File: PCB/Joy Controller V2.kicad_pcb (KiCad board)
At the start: 2 copper layers, 182.7 x 66.7 mm, 24 parts, among them J1 Conn_02x16_Odd_Even, J2 JOY1, J3 JOY2, J4 USB_C_Receptacle_USB2.0_16P, SW1 SW_Push, SW10 SW_Push, SW12 RotaryEncoder_Switch_MP, SW2 SW_Push, SW3 SW_Push, SW4 SW_Push, SW5 SW_Push, SW6 SW_Push, SW7 SW_Push, SW8 SW_Push

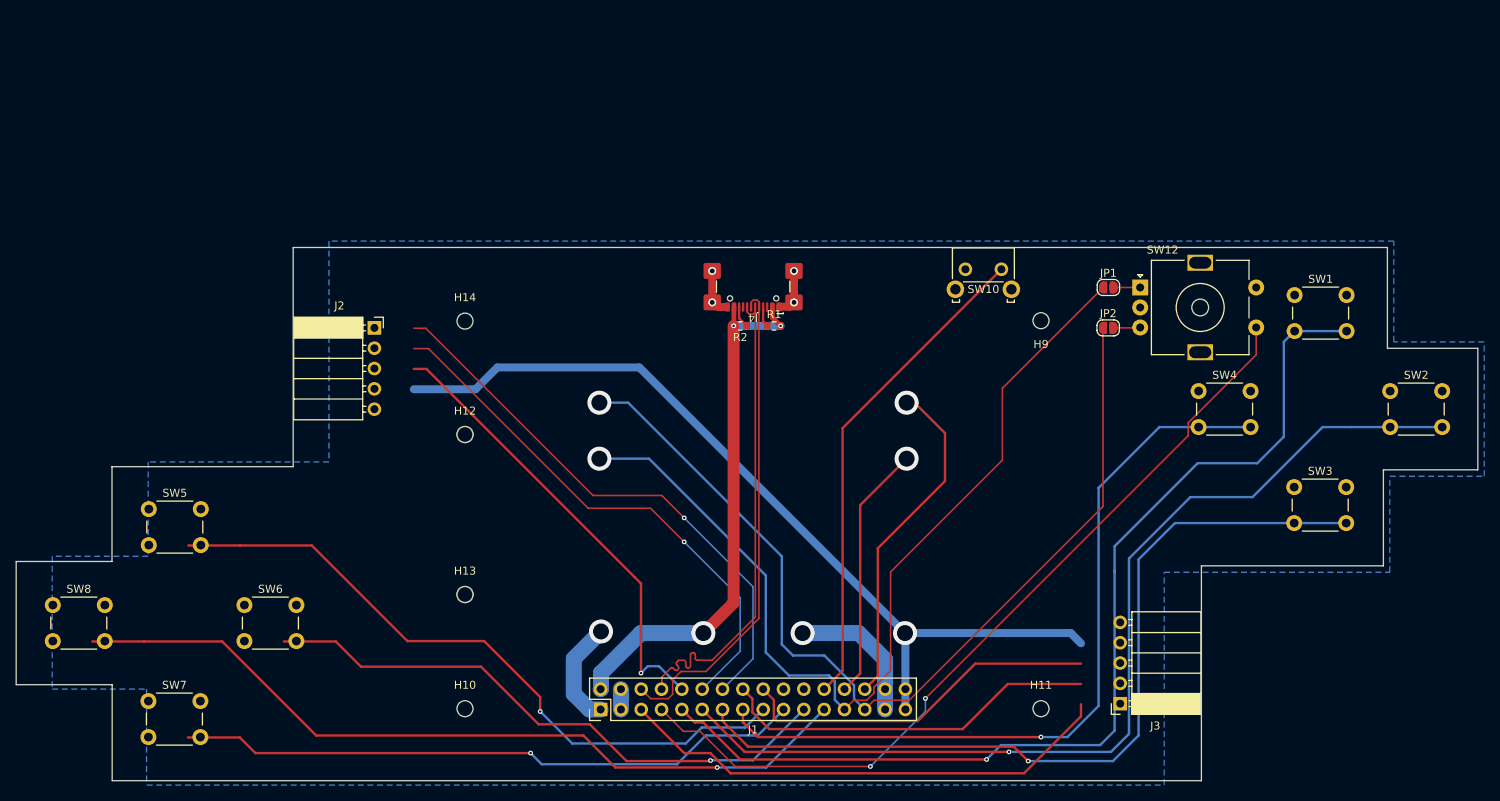
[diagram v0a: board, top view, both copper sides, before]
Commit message: Add files via upload
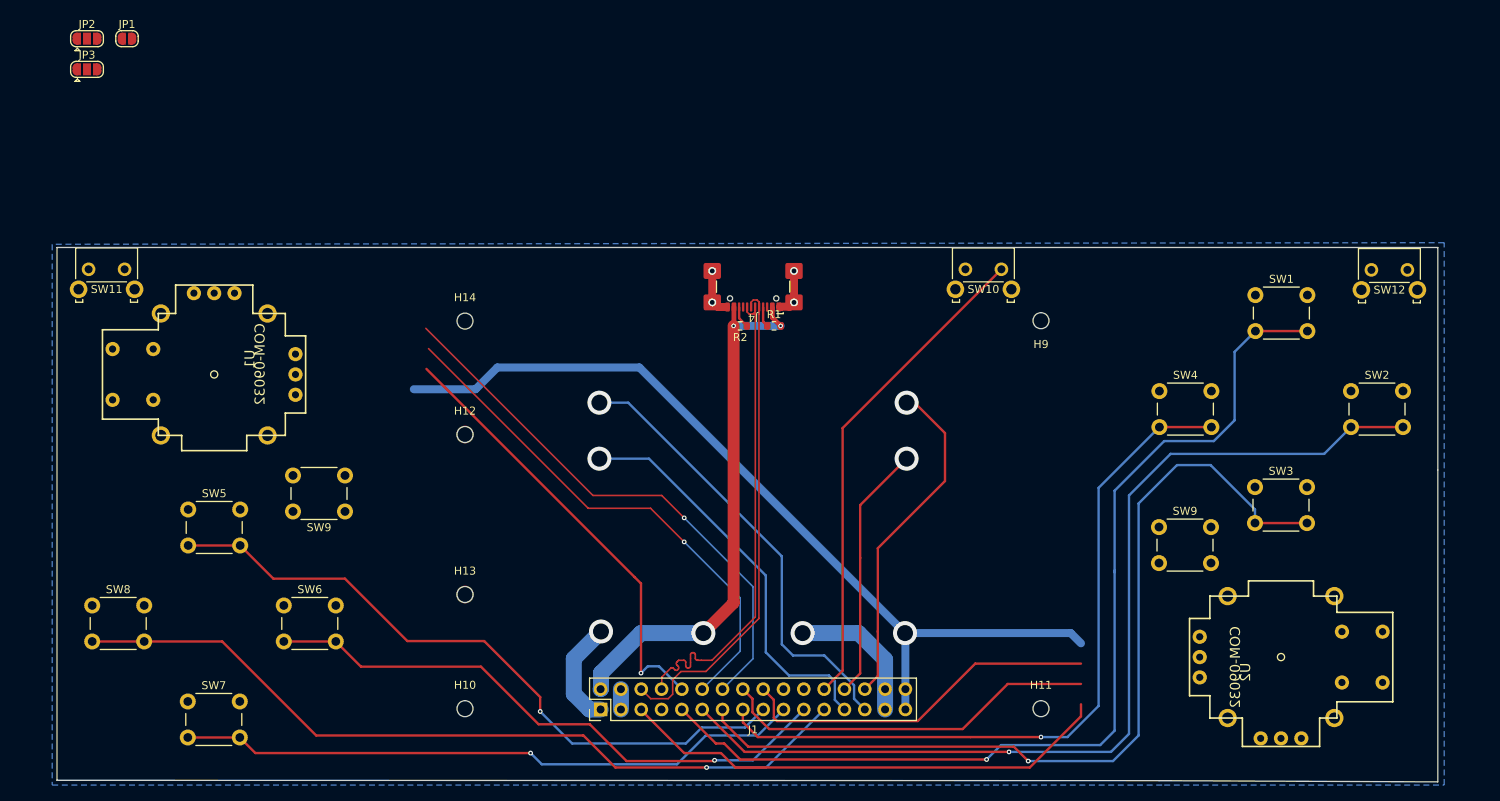
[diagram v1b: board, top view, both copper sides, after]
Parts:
- removed J2: JOY1, Connector_PinSocket_2.54mm:PinSocket_1x05_P2.54mm_Horizontal
- removed J3: JOY2, Connector_PinSocket_2.54mm:PinSocket_1x05_P2.54mm_Horizontal
- added JP3: SolderJumper_3_Open, Jumper:SolderJumper-3_P1.3mm_Open_RoundedPad1.0x1.5mm, F.Cu at (46.4, 42.7)
- added SW11: SW_Push, Button_Switch_THT:SW_Tactile_SKHH_Angled, F.Cu at (46.5, 67.7)
- added SW9: SW_Push, Button_Switch_THT:SW_PUSH_6mm, F.Cu at (180.3, 100.0)
- added SW9: SW_Push, Button_Switch_THT:SW_PUSH_6mm, F.Cu at (78.6, 98.0)
- added U1: COM-09032, Joy:JOYSTICK, B.Cu at (62.2, 80.9)
- added U2: COM-09032, Joy:JOYSTICK, B.Cu at (195.6, 116.2)
- JP1: value SolderJumper_2_Bridged -> SolderJumper_2_Open
- JP2: value SolderJumper_2_Bridged -> SolderJumper_3_Open; footprint Jumper:SolderJumper-2_P1.3mm_Open_RoundedPad1.0x1.5mm -> Jumper:SolderJumper-3_P1.3mm_Open_RoundedPad1.0x1.5mm
- SW12: value RotaryEncoder_Switch_MP -> SW_Push; footprint Rotary_Encoder:RotaryEncoder_Alps_EC11E-Switch_Vertical_H20mm_MountingHoles -> Button_Switch_THT:SW_Tactile_SKHH_Angled
- moved JP2 132.7 mm to (46.4, 38.9)
- moved JP1 126.6 mm to (51.4, 38.9)
- moved SW12 29.0 mm to (206.9, 67.8)
- moved SW7 4.93 mm to (59.0, 121.8)
- moved SW5 4.93 mm to (59.0, 97.8)
- moved SW6 4.93 mm to (71.0, 109.8)
- moved SW8 4.93 mm to (47.0, 109.8)
- moved SW1 4.90 mm to (192.4, 71.0)
- moved SW2 4.90 mm to (204.3, 83.0)
- moved SW3 4.90 mm to (192.3, 95.0)
- moved SW4 4.90 mm to (180.4, 83.0)
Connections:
- JP1 pad 1: RXD(GPIO44) -> Net-(JP1-A)
- JP1 pad 2: Net-(JP1-B) -> BOOT(GPIO0)
- JP2 pad 1: TXD(GPIO43) -> Net-(JP2-A)
- JP2 pad 2: Net-(JP2-B) -> RXD(GPIO44)
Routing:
- net GPIO38: track 103.9 -> 0.00 mm, vias 2 -> 0
- net RXD(GPIO44): track 117.7 -> 50.6 mm
- net TXD(GPIO43): track 119.1 -> 56.5 mm
- net GPIO41: track 106.7 -> 112.9 mm
- net GPIO42: track 97.8 -> 92.9 mm
- net Net-(JP2-B): track 3.37 -> 0.00 mm
- net Net-(JP1-B): track 3.32 -> 0.00 mm
- net GPIO39: track 128.5 -> 125.7 mm
- net GPIO10: track 67.1 -> 65.2 mm
- net GPIO11: track 57.4 -> 55.8 mm
- net GPIO9: track 70.2 -> 68.7 mm
- net GPIO21: track 62.8 -> 62.2 mm
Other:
- board size 182.7 x 66.7 mm -> 172.6 x 66.8 mm
